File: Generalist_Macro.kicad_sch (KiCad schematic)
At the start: 7 parts, among them SW1 SW_Push, SW2 SW_Push, SW3 SW_Push, SW4 SW_Push, U1 XIAO-RP2040-DIP

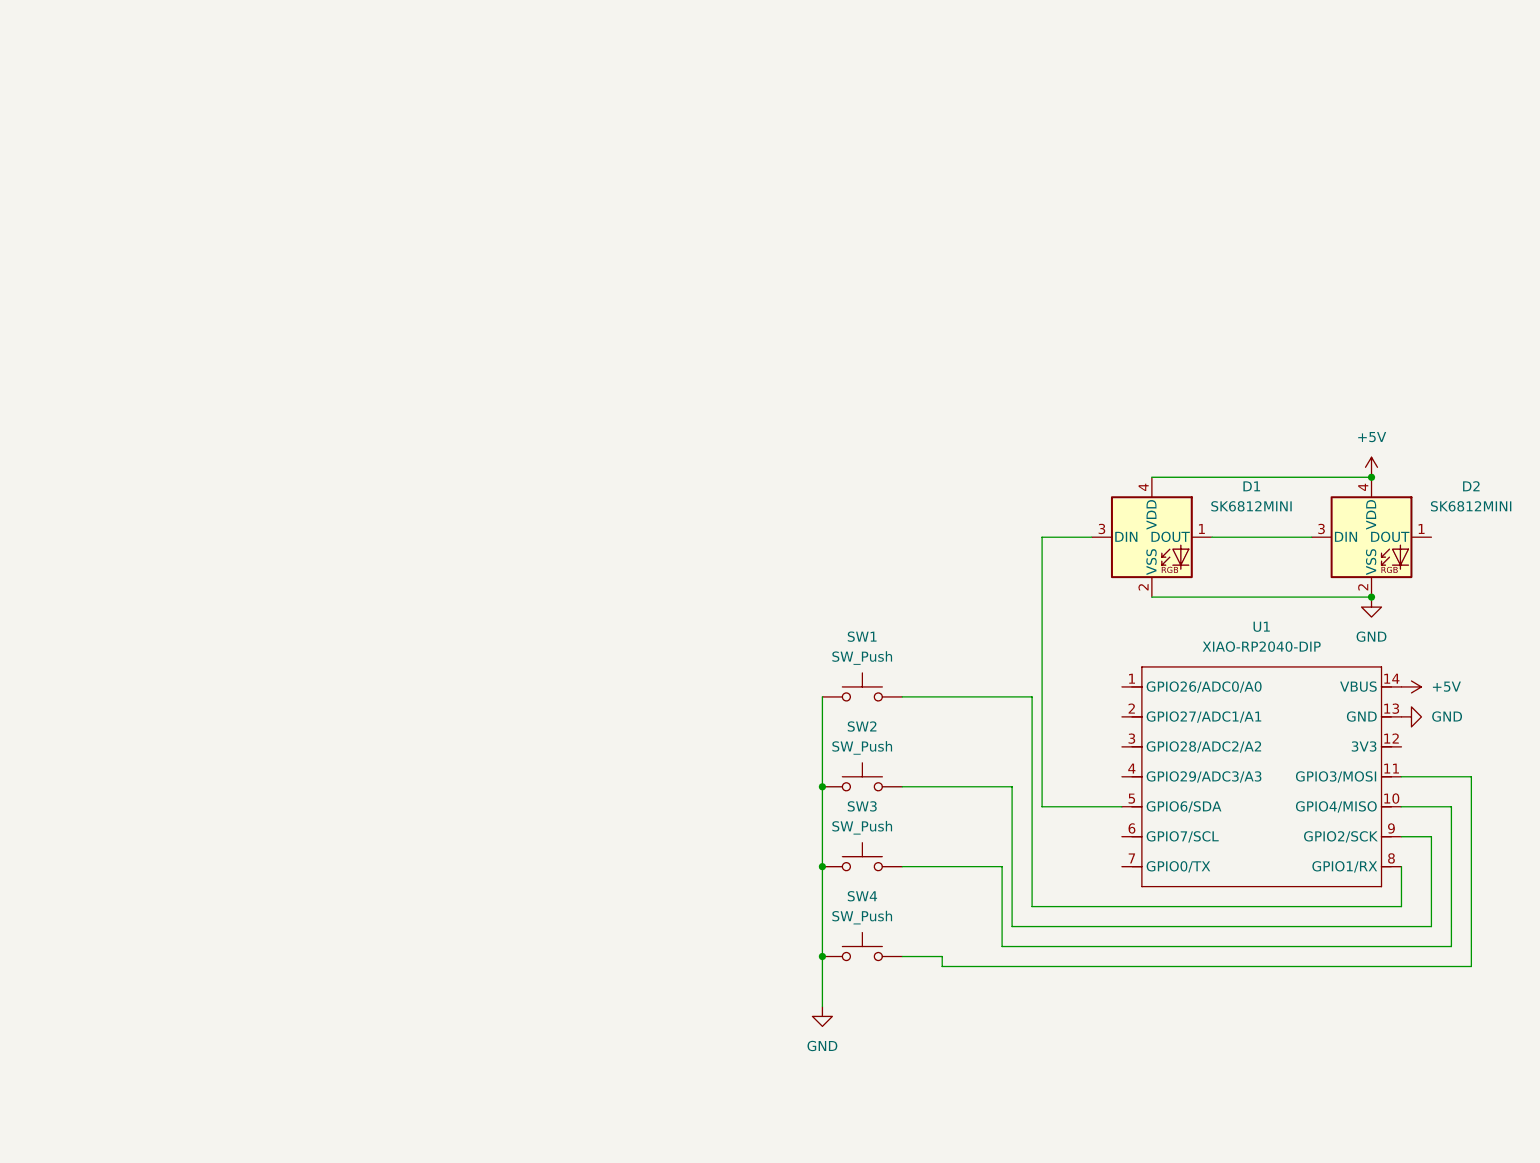
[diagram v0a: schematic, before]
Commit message: Finished Schematic, Started PCB
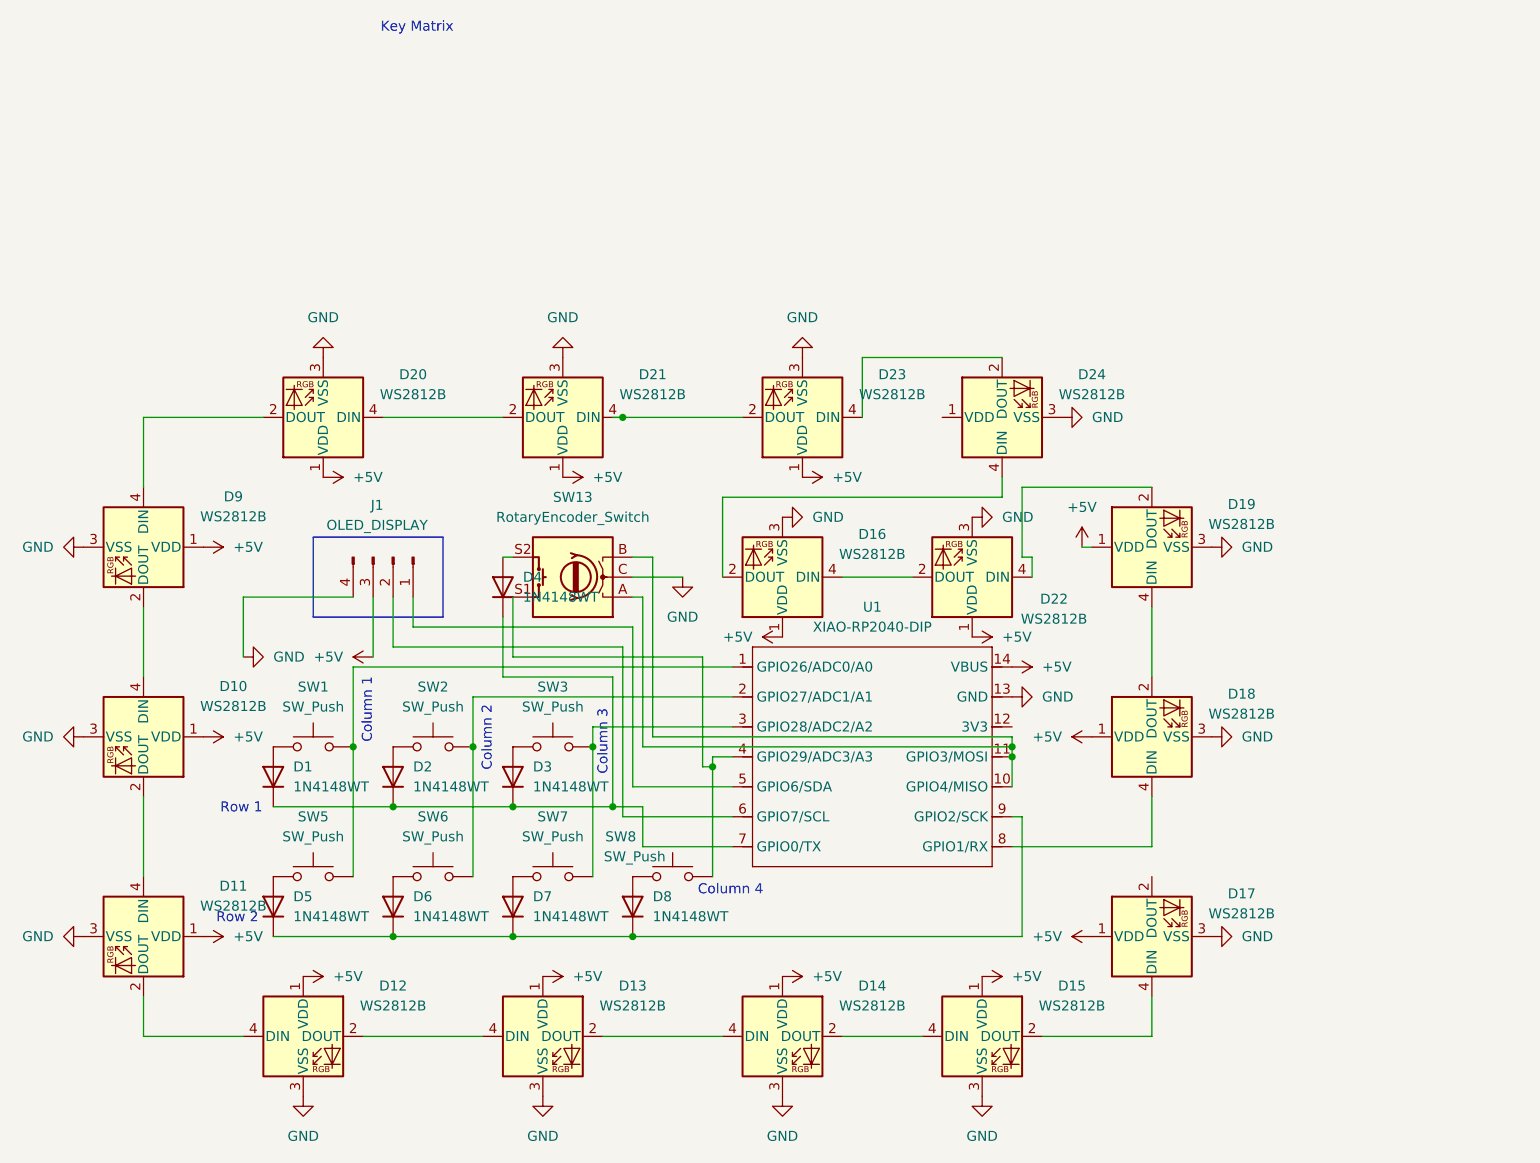
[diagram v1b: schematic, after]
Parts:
- removed D1, D2: SK6812MINI, LED_SMD:LED_SK6812MINI_PLCC4_3.5x3.5mm_P1.75mm, symbol LED:SK6812MINI
- removed SW4: SW_Push, Button_Switch_Keyboard:SW_Cherry_MX_1.00u_PCB, symbol Switch:SW_Push
- added D1, D2, D3, D4, D5, D6, D7, D8: 1N4148WT, Diode_SMD:D_SOD-523, symbol Diode:1N4148WT
- added D10, D11, D12, D13, D14, D15, D16, D17, D18, D19, D20, D21, D22, D23, D24, D9: WS2812B, LED_SMD:LED_WS2812B_PLCC4_5.0x5.0mm_P3.2mm, symbol LED:WS2812B
- added J1: OLED_DISPLAY, Connector_PinHeader_2.54mm:PinHeader_1x04_P2.54mm_Vertical, symbol Connector:Conn_01x04_Pin
- added SW13: RotaryEncoder_Switch, Rotary_Encoder:RotaryEncoder_Alps_EC11E-Switch_Vertical_H20mm, symbol Device:RotaryEncoder_Switch
- added SW5, SW6, SW7, SW8: SW_Push, Button_Switch_Keyboard:SW_Cherry_MX_1.00u_PCB, symbol Switch:SW_Push
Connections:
- net +5V: now also D10.1 (VDD), D11.1 (VDD), D12.1 (VDD), D13.1 (VDD), D14.1 (VDD), D15.1 (VDD), D16.1 (VDD), D17.1 (VDD), D18.1 (VDD), D19.1 (VDD), D20.1 (VDD), D21.1 (VDD), D22.1 (VDD), D23.1 (VDD), D9.1 (VDD), J1.3 (Pin_3)
- net GND: now also D10.3 (VSS), D11.3 (VSS), D12.3 (VSS), D13.3 (VSS), D14.3 (VSS), D15.3 (VSS), D16.3 (VSS), D17.3 (VSS), D18.3 (VSS), D19.3 (VSS), D20.3 (VSS), D21.3 (VSS), D22.3 (VSS), D23.3 (VSS), D24.3 (VSS), D9.3 (VSS), J1.4 (Pin_4), SW13.C; no longer SW1.1, SW2.1, SW3.1
- net at U1.5 (GPIO6/SDA): now also J1.1 (Pin_1)
- net at U1.11 (GPIO3/MOSI): now also U1.10 (GPIO4/MISO), SW13.A, SW13.B
- net at SW3.2: now also U1.3 (GPIO28/ADC2/A2), SW7.2; no longer U1.10 (GPIO4/MISO)
- net at SW1.2: now also U1.1 (GPIO26/ADC0/A0), SW5.2; no longer U1.8 (GPIO1/RX)
- net at U1.2 (GPIO27/ADC1/A1): now also SW2.2, SW6.2
- net at U1.4 (GPIO29/ADC3/A3): now also SW13.S1, SW8.2
- net at U1.6 (GPIO7/SCL): now also J1.2 (Pin_2)
- net at U1.7 (GPIO0/TX): now also D1.1 (K), D2.1 (K), D3.1 (K), D4.1 (K)
- net at U1.9 (GPIO2/SCK): now also D5.1 (K), D6.1 (K), D7.1 (K), D8.1 (K); no longer SW2.2
- new net: D5.2 (A), SW5.1
- new net: D20.2 (DOUT), D9.4 (DIN)
- new net: D20.4 (DIN), D21.2 (DOUT)
- new net: D15.2 (DOUT), D17.4 (DIN)
- new net: D14.2 (DOUT), D15.4 (DIN)
- new net: D13.2 (DOUT), D14.4 (DIN)
- new net: D3.2 (A), SW3.1
- new net: D10.4 (DIN), D9.2 (DOUT)
- new net: D21.4 (DIN), D23.2 (DOUT)
- new net: D1.2 (A), SW1.1
- new net: D2.2 (A), SW2.1
- new net: D10.2 (DOUT), D11.4 (DIN)
- new net: D12.2 (DOUT), D13.4 (DIN)
- new net: D11.2 (DOUT), D12.4 (DIN)
- new net: D6.2 (A), SW6.1
- new net: D19.2 (DOUT), D22.4 (DIN)
- new net: D18.2 (DOUT), D19.4 (DIN)
- new net: D16.4 (DIN), D22.2 (DOUT)
- new net: D23.4 (DIN), D24.2 (DOUT)
- new net: D16.2 (DOUT), D24.4 (DIN)
- new net: D8.2 (A), SW8.1
- new net: D4.2 (A), SW13.S2
- new net: D7.2 (A), SW7.1
- new net: D18.4 (DIN), U1.8 (GPIO1/RX)
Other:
- note added: "Column 1"
- note added: "Column 2"
- note added: "Column 3"
- note added: "Column 4"
- note added: "Key Matrix"
- note added: "Row 1"
- note added: "Row 2"
- moved on the sheet: SW1, U1
